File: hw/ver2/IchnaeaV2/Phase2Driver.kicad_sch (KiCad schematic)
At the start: 21 parts, among them Q6 MCAC80N10Y, Q7 MCAC80N10Y, Q8 MCAC80N10Y, Q9 MCAC80N10Y, U3 HIP2210

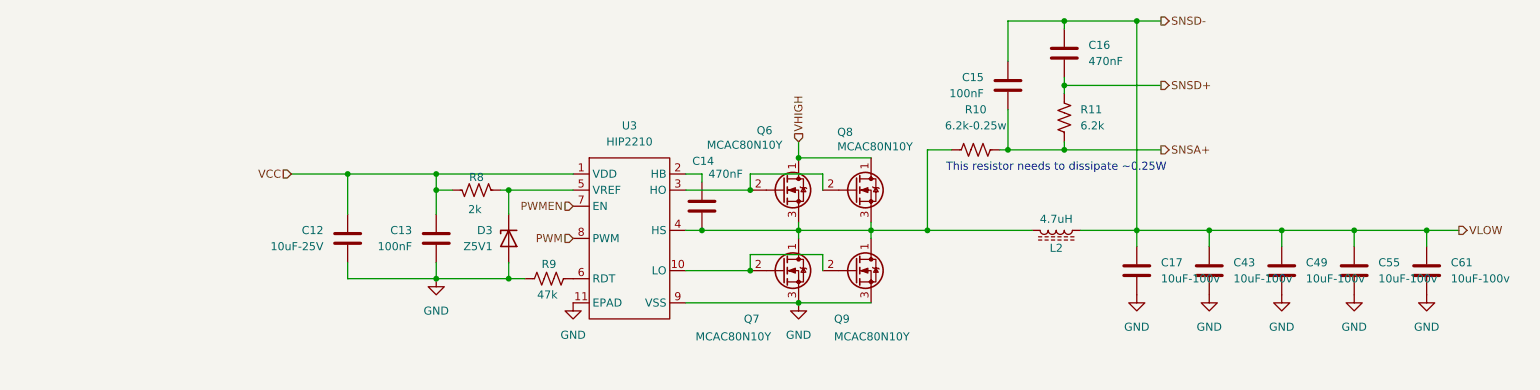
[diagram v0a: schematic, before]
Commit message: Sync work to main PC
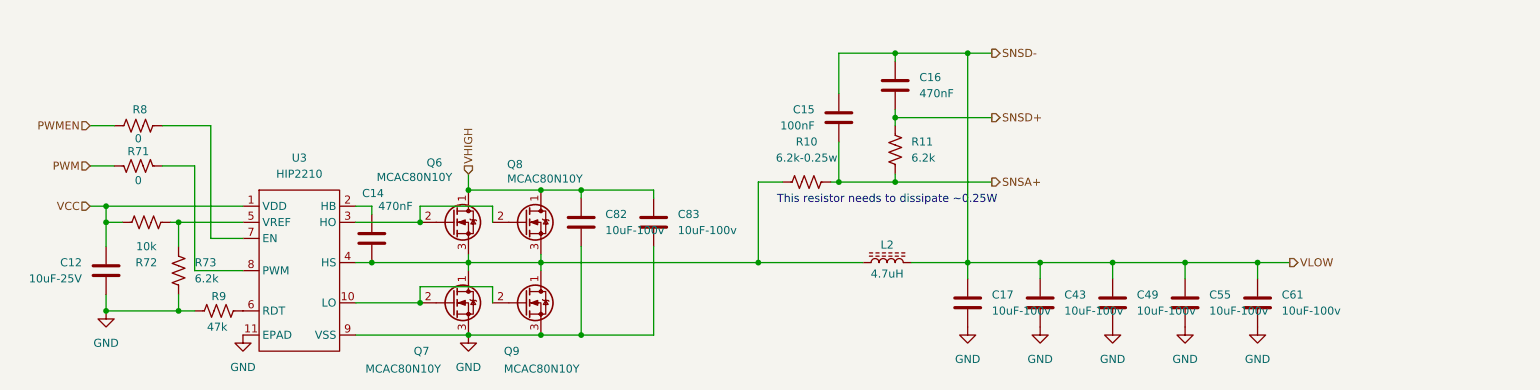
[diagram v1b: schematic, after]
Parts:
- removed C13: 100nF, Capacitor_SMD:C_0603_1608Metric, symbol Device:C
- removed D3: Z5V1, Diode_SMD:D_SOD-123, symbol Device:D_Zener
- added C82, C83: 10uF-100v, Capacitor_SMD:C_1210_3225Metric_Pad1.33x2.70mm_HandSolder, symbol Device:C
- added R71: 0, Resistor_SMD:R_0603_1608Metric, symbol Device:R_US
- added R72: 10k, Resistor_SMD:R_0603_1608Metric, symbol Device:R_US
- added R73: 6.2k, Resistor_SMD:R_0603_1608Metric, symbol Device:R_US
- R8: value 2k -> 0; LCSC (none) -> C21189
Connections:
- net GND: now also C82.2, C83.2, R73.2
- net PWM: now also R71.2; no longer U3.8 (PWM)
- net PWMEN: now also R8.2; no longer U3.7 (EN)
- net SNSD-: now also L2.2; no longer L2.1
- net VCC: now also R72.1; no longer R8.2
- net VHIGH: now also C82.1, C83.1
- net at C14.2, Q6.3 (S), Q7.1 (D)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: now also L2.1; no longer L2.2
- net at R8.1: now also U3.7 (EN); no longer U3.5 (VREF)
- new net: R71.1, U3.8 (PWM)
- new net: R72.2, R73.1, U3.5 (VREF)
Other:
- moved on the sheet: C12, C14, C15, C16, C17, C43, C49, C55, C61, L2, Q6, Q7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
